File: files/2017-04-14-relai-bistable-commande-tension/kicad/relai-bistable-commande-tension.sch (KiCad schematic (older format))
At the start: 19 parts, among them T1 BC337, T2 BC337

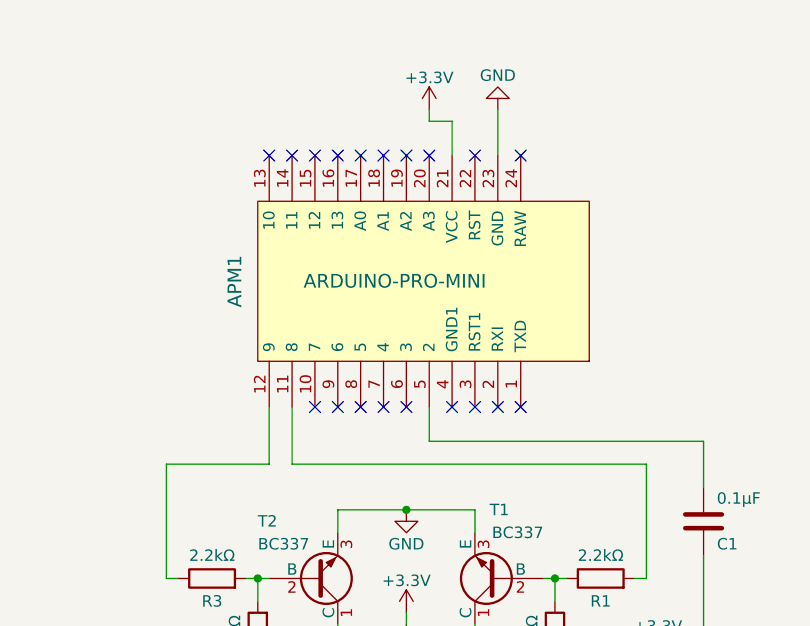
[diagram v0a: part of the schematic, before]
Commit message: modif PCB Kicad
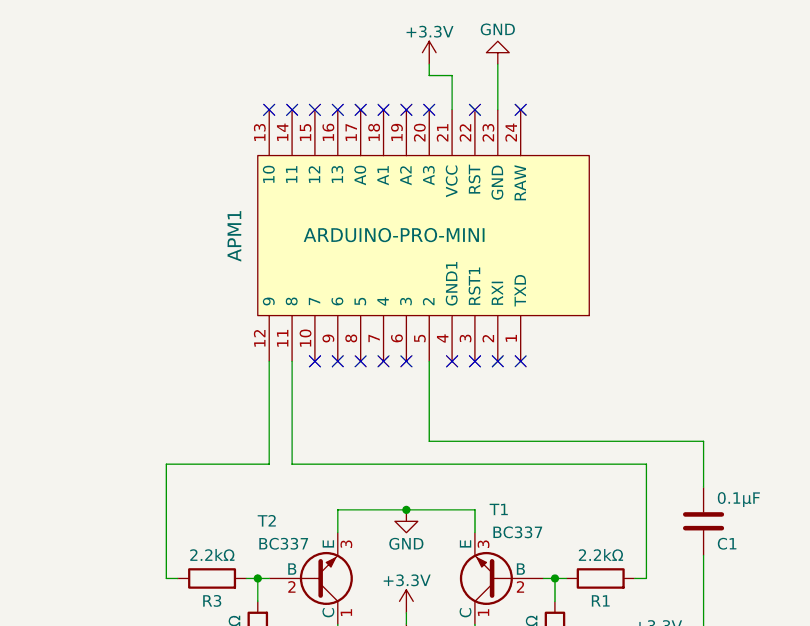
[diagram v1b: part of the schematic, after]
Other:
- moved on the sheet: APM1
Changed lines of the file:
@@
 L ARDUINO-PRO-MINI APM1
 U 1 1 58F25AB8
-P 3900 2050
-F 0 "APM1" H 3900 500 60  0000 C CNN
-F 1 "ARDUINO-PRO-MINI" V 3900 1200 60  0000 C CNN
-F 2 "empreintes:Arduino_Pro_Mini" H 3900 2050 60  0001 C CNN
-F 3 "" H 3900 2050 60  0001 C CNN
-	1    3900 2050
+P 3900 1850
+F 0 "APM1" H 3900 300 60  0000 C CNN
+F 1 "ARDUINO-PRO-MINI" V 3900 1000 60  0000 C CNN
+F 2 "empreintes:Arduino_Pro_Mini" H 3900 1850 60  0001 C CNN
+F 3 "" H 3900 1850 60  0001 C CNN
+	1    3900 1850
 	0    1    -1   0
 $EndComp
@@
 L GND #PWR05
 U 1 1 58F26E0D
-P 3500 1300
-F 0 "#PWR05" H 3500 1050 50  0001 C CNN
-F 1 "GND" H 3500 1150 50  0000 C CNN
-F 2 "" H 3500 1300 50  0000 C CNN
-F 3 "" H 3500 1300 50  0000 C CNN
-	1    3500 1300
+P 3500 1100
+F 0 "#PWR05" H 3500 850 50  0001 C CNN
+F 1 "GND" H 3500 950 50  0000 C CNN
+F 2 "" H 3500 1100 50  0000 C CNN
+F 3 "" H 3500 1100 50  0000 C CNN
+	1    3500 1100
 	-1   0    0    1
 $EndComp
@@
 L +3.3V #PWR06
 U 1 1 58F26E82
-P 3200 1300
-F 0 "#PWR06" H 3200 1150 50  0001 C CNN
-F 1 "+3.3V" H 3200 1440 50  0000 C CNN
-F 2 "" H 3200 1300 50  0000 C CNN
-F 3 "" H 3200 1300 50  0000 C CNN
-	1    3200 1300
+P 3200 1100
+F 0 "#PWR06" H 3200 950 50  0001 C CNN
+F 1 "+3.3V" H 3200 1240 50  0000 C CNN
+F 2 "" H 3200 1100 50  0000 C CNN
+F 3 "" H 3200 1100 50  0000 C CNN
+	1    3200 1100
 	1    0    0    -1
 $EndComp
@@
 	1    0    0    -1
 $EndComp
-NoConn ~ 2500 1500
-NoConn ~ 2600 1500
-NoConn ~ 2700 1500
-NoConn ~ 2800 1500
-NoConn ~ 2900 1500
-NoConn ~ 3000 1500
-NoConn ~ 3100 1500
-NoConn ~ 3200 1500
-NoConn ~ 3400 1500
-NoConn ~ 3600 1500
-NoConn ~ 3600 2600
-NoConn ~ 3500 2600
-NoConn ~ 3400 2600
-NoConn ~ 3300 2600
-NoConn ~ 3100 2600
-NoConn ~ 3000 2600
-NoConn ~ 2900 2600
-NoConn ~ 2800 2600
-NoConn ~ 2700 2600
+NoConn ~ 2500 1300
+NoConn ~ 2600 1300
+NoConn ~ 2700 1300
+NoConn ~ 2800 1300
+NoConn ~ 2900 1300
+NoConn ~ 3000 1300
+NoConn ~ 3100 1300
+NoConn ~ 3200 1300
+NoConn ~ 3400 1300
+NoConn ~ 3600 1300
+NoConn ~ 3600 2400
+NoConn ~ 3500 2400
+NoConn ~ 3400 2400
+NoConn ~ 3100 2400
+NoConn ~ 3000 2400
+NoConn ~ 2800 2400
+NoConn ~ 2700 2400
 $Comp
 L ALIM-IRM-03-3.3 ALIM1
@@
 	2500 2850 2050 2850
 Wire Wire Line
-	3200 2600 3200 2750
-Wire Wire Line
 	4400 2750 4400 2950
 Wire Wire Line
 	4150 2850 2600 2850
 Wire Wire Line
-	2600 2850 2600 2600
-Wire Wire Line
-	2500 2850 2500 2600
-Wire Wire Line
-	3500 1500 3500 1300
-Wire Wire Line
-	3300 1500 3300 1350
-Wire Wire Line
-	3300 1350 3200 1350
-Wire Wire Line
-	3200 1350 3200 1300
+	3500 1300 3500 1100
+Wire Wire Line
+	3300 1300 3300 1150
+Wire Wire Line
+	3300 1150 3200 1150
+Wire Wire Line
+	3200 1150 3200 1100
 Wire Wire Line
 	4200 3700 4200 3750
@@
 Wire Wire Line
 	2650 5450 2650 5200
+NoConn ~ 2900 2400
+Wire Wire Line
+	2500 2850 2500 2400
+Wire Wire Line
+	2600 2850 2600 2400
+Wire Wire Line
+	3200 2400 3200 2750
+NoConn ~ 3300 2400
 $EndSCHEMATC
